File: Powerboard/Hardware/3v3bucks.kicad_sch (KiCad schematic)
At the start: 44 parts, among them IC1 SiC437BED-T1-GE3, IC2 SiC437BED-T1-GE3, Q5 SSM6J511NU,LF, Q6 SSM6J511NU,LF, U8 LTC4412xS6, U9 LTC4412xS6

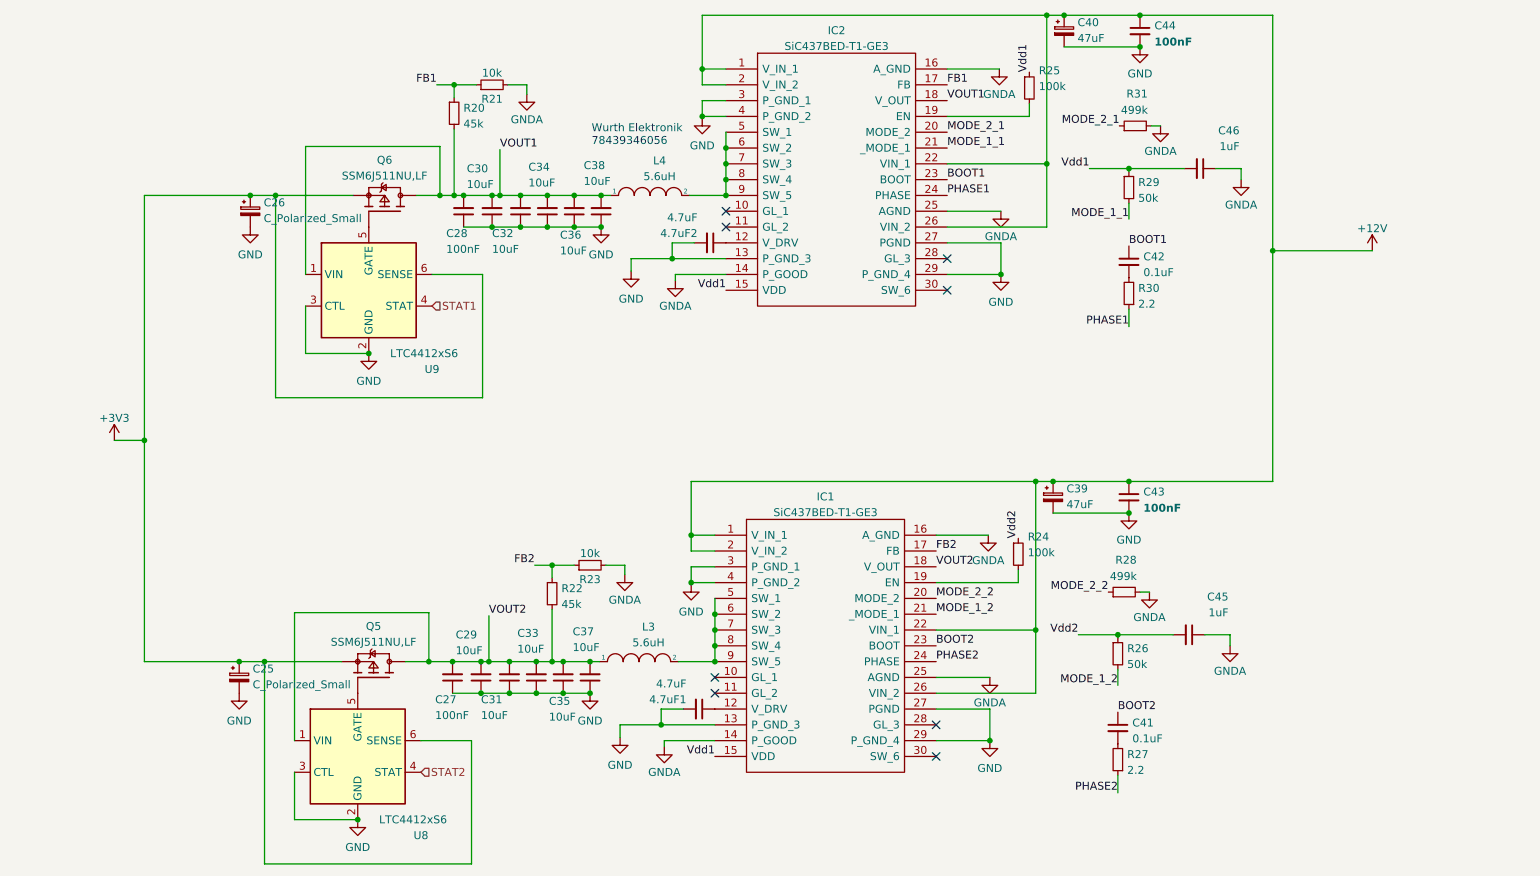
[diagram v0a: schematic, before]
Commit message: latest
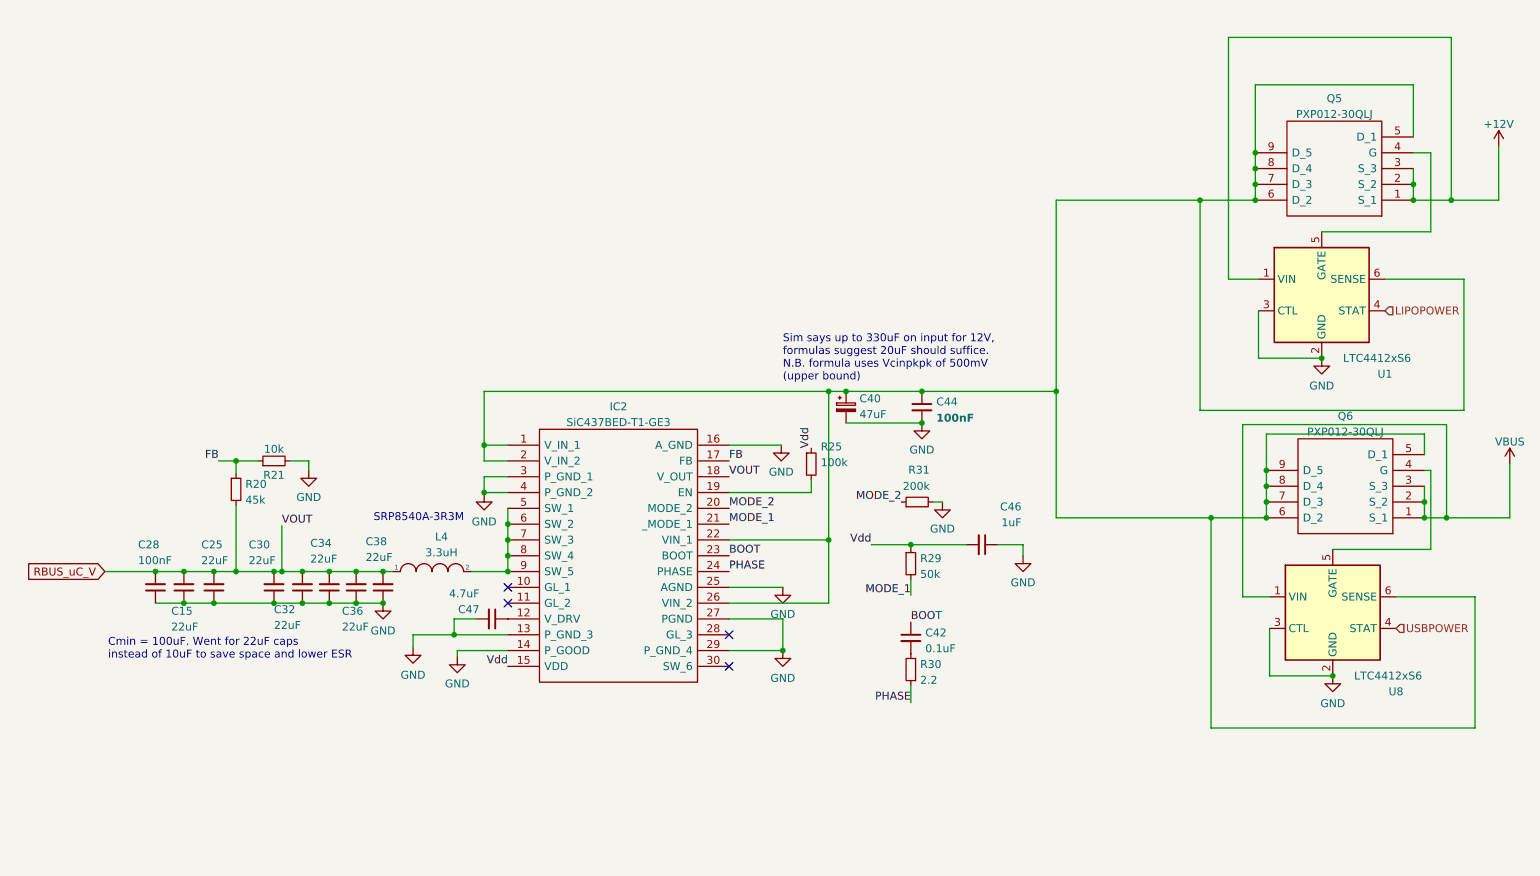
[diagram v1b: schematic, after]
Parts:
- removed 4.7uF1: 4.7uF, Capacitor_SMD:C_0402_1005Metric, symbol Device:C_Small
- removed C25, C26: C_Polarized_Small, Capacitor_SMD:CP_Elec_10x10, symbol Device:C_Polarized_Small
- removed C27: 100nF, symbol Device:C_Small
- removed C29, C31, C33, C35, C37: 10uF, Resistor_SMD:R_0805_2012Metric, symbol Device:C_Small
- removed C39: 47uF, Capacitor_SMD:CP_Elec_8x11.9, symbol Device:C_Polarized_Small
- removed C41: 0.1uF, Capacitor_SMD:C_0402_1005Metric, symbol Device:C_Small
- removed C43: 100nF, Resistor_SMD:R_1206_3216Metric, symbol Device:C_Small
- removed C45: 1uF, Capacitor_SMD:C_0402_1005Metric, symbol Device:C_Small
- removed IC1: SiC437BED-T1-GE3, iclr:SiC437BEDT1GE3, symbol iclr:SiC437BED-T1-GE3
- removed L3: 5.6uH, Inductor_SMD:L_6.3x6.3_H3, symbol pspice:INDUCTOR
- removed Q5, Q6: SSM6J511NU,LF, iclr:TRANS_SSM6J511NU,LF, symbol iclr:SSM6J511NU,LF
- removed R22: 45k, Resistor_SMD:R_0402_1005Metric, symbol Device:R_Small
- removed R23: 10k, Resistor_SMD:R_0402_1005Metric, symbol Device:R_Small
- removed R24: 100k, Resistor_SMD:R_0402_1005Metric, symbol Device:R_Small
- removed R26: 50k, Resistor_SMD:R_0402_1005Metric, symbol Device:R_Small
- removed R27: 2.2, Resistor_SMD:R_0402_1005Metric, symbol Device:R_Small
- removed R28: 499k, Resistor_SMD:R_0402_1005Metric, symbol Device:R_Small
- removed U9: LTC4412xS6, Package_TO_SOT_SMD:TSOT-23-6, symbol Power_Management:LTC4412xS6
- added C15, C25: 22uF, Capacitor_SMD:C_0603_1608Metric, symbol Device:C_Small
- added Q5, Q6: PXP012-30QLJ, iclr:PXP01230QLJ, symbol iclr:PXP012-30QLJ
- added U1: LTC4412xS6, Package_TO_SOT_SMD:TSOT-23-6, symbol Power_Management:LTC4412xS6
- C28: footprint (none) -> Capacitor_SMD:C_0402_1005Metric
- C30, C32, C34, C36, C38: value 10uF -> 22uF; footprint Resistor_SMD:R_0805_2012Metric -> Capacitor_SMD:C_0603_1608Metric
- C40: footprint Capacitor_SMD:CP_Elec_8x11.9 -> Capacitor_Tantalum_SMD:CP_EIA-7343-31_Kemet-D
- C44: footprint Resistor_SMD:R_1206_3216Metric -> Capacitor_SMD:C_0603_1608Metric
- L4: value 5.6uH -> 3.3uH; footprint Inductor_SMD:L_6.3x6.3_H3 -> Inductor_SMD:L_10.4x10.4_H4.8
- R31: value 499k -> 200k
- renumbered 4.7uF2 to C47
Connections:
- net GNDA is gone; now on net GND: C46.1, IC2.14 (P_GOOD), IC2.16 (A_GND), IC2.25 (AGND), R21.2, R31.2
- net +12V: now also Q5.1 (S_1), Q5.2 (S_2), Q5.3 (S_3), U1.1 (VIN); no longer C40.1, C44.1, IC2.1 (V_IN_1), IC2.2 (V_IN_2), IC2.22 (VIN_1), IC2.26 (VIN_2)
- net GND: now also C15.1, C25.1, U1.2 (GND), U1.3 (CTL)
- net at U8.5 (GATE): now also Q6.4 (G)
- net +3V3: no longer names the net of U8.6 (SENSE)
- net +3V3: now also C40.1, C44.1, IC2.1 (V_IN_1), IC2.2 (V_IN_2), IC2.22 (VIN_1), IC2.26 (VIN_2), Q5.5 (D_1), Q5.6 (D_2), Q5.7 (D_3), Q5.8 (D_4), Q5.9 (D_5), Q6.5 (D_1), Q6.6 (D_2), Q6.7 (D_3), Q6.8 (D_4), Q6.9 (D_5), U1.6 (SENSE)
- net BOOT1 renamed BOOT
- net FB1 renamed FB
- net MODE_1_1 renamed MODE_1
- net MODE_2_1 renamed MODE_2
- net PHASE1 renamed PHASE
- net STAT2 renamed USBPOWER
- net VOUT1 renamed RBUS_uC_V
- net RBUS_uC_V: now also C15.2, C25.2
- net VOUT2 renamed VBUS
- net VBUS: now also Q6.1 (S_1), Q6.2 (S_2), Q6.3 (S_3)
- net Vdd1 renamed Vdd
- new net: Q5.4 (G), U1.5 (GATE)
- new net LIPOPOWER: U1.4 (STAT)
- no-connect marks 8 -> 4
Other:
- note added: "Cmin = 100uF. Went for 22uF caps instead of 10uF to save space and lower ESR"
- note added: "SRP8540A-3R3M"
- note added: "Sim says up to 330uF on input for 12V, formulas suggest 20uF should suffice. N.B. formula uses Vcinpkpk of 500mV (upper bound)"
- note removed: "Wurth Elektronik 78439346056"
- moved on the sheet: C28, C30, C32, C34, C36, C38, C40, C42, C44, C46, C47, IC2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
